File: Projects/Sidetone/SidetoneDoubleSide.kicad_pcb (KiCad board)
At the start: 2 copper layers, 85.5 x 84.8 mm, 54 parts, among them Q1 2N3904, Q2 2N3904, Q3 2N3904, SW1 morse key, SW2 On/off, U1 4N35, U2 LM324, U3 LM386

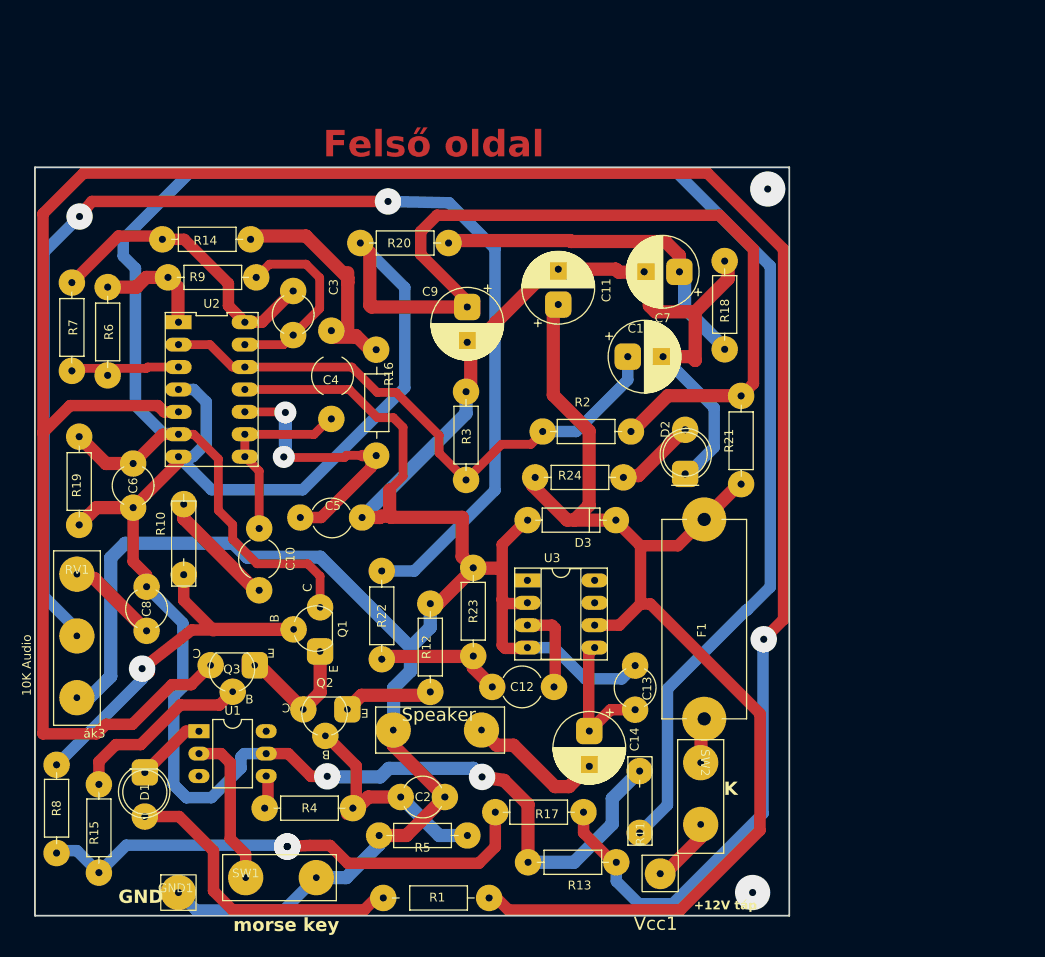
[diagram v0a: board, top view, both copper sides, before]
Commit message: 20240226 sidetone last update
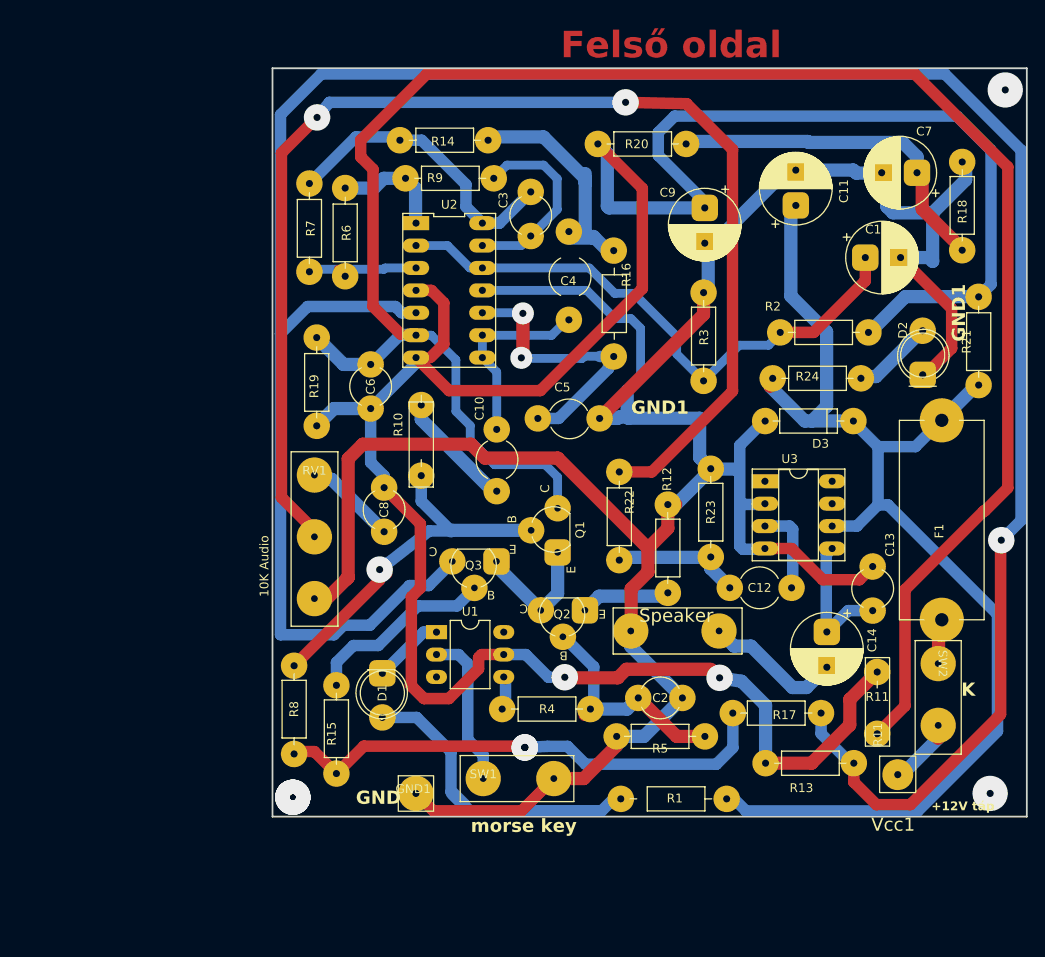
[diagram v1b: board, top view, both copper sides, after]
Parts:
- moved Q3 29.8 mm to (140.3, 107.2)
- moved C11 29.2 mm to (174.3, 66.9)
- moved C12 29.2 mm to (166.8, 110.2)
- moved C14 29.2 mm to (177.8, 115.2)
- moved C2 29.2 mm to (156.4, 122.7)
- moved C9 29.2 mm to (164.0, 67.2)
- moved GND1 29.2 mm to (131.2, 133.5)
- moved R10 29.2 mm to (131.8, 97.5)
- moved R11 29.2 mm to (183.5, 119.8)
- moved R13 29.2 mm to (170.8, 130.1)
- moved R15 29.2 mm to (122.2, 131.3)
- moved R17 29.2 mm to (177.1, 124.4)
- moved R18 29.2 mm to (193.1, 72.0)
- moved R21 29.2 mm to (195.0, 77.2)
- moved R23 29.2 mm to (164.6, 106.7)
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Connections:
- C1 pad 1: Net-(U2A--) -> GNDD
- C10 pad 1: Net-(U2C--) -> GNDD
- C10 pad 2: Net-(C10-Pad2) -> GNDD
- C11 pad 1: Net-(D3-K) -> GNDD
- C12 pad 1: Net-(C12-Pad1) -> GNDD
- C12 pad 2: Net-(U3-+) -> GNDD
- C13 pad 1: Net-(C13-Pad1) -> GNDD
- C14 pad 1: Net-(C13-Pad1) -> GNDD
- C2 pad 1: Net-(Q2-B) -> GNDD
- C3 pad 1: Net-(C3-Pad1) -> GNDD
- C4 pad 1: Net-(U2C--) -> GNDD
- C5 pad 1: Net-(U2C-+) -> GNDD
- C6 pad 1: Net-(Q1-C) -> GNDD
- C6 pad 2: Net-(U2E-V+) -> GNDD
- C7 pad 1: Net-(C7-Pad1) -> GNDD
- C8 pad 1: Net-(U2E-V+) -> GNDD
- C8 pad 2: Net-(C8-Pad2) -> GNDD
- C9 pad 1: Net-(U2E-V+) -> GNDD
- D1 pad 1: Net-(D1-K) -> GNDD
- D1 pad 2: Net-(D1-A) -> GNDD
- D3 pad 1: Net-(D3-K) -> GNDD
- F1 pad 1: Net-(D3-K) -> GNDD
- Q1 pad 2: Net-(Q1-B) -> GNDD
- Q1 pad 3: Net-(Q1-C) -> GNDD
- Q2 pad 1: Net-(Q2-E) -> GNDD
- Q2 pad 2: Net-(Q2-B) -> GNDD
- Q3 pad 2: Net-(Q3-B) -> GNDD
- Q3 pad 3: Net-(Q3-C) -> GNDD
- R1 pad 1: Net-(D1-A) -> GNDD
- R1 pad 2: Net-(D3-K) -> GNDD
- R10 pad 1: Net-(Q1-B) -> GNDD
- R10 pad 2: Net-(C10-Pad2) -> GNDD
- R11 pad 1: Net-(U2E-V+) -> GNDD
- R11 pad 2: Net-(Q1-C) -> GNDD
- R12 pad 1: Net-(Q2-E) -> GNDD
- R13 pad 1: Net-(U2E-V+) -> GNDD
- R13 pad 2: Net-(Q3-C) -> GNDD
- R14 pad 1: Net-(C3-Pad1) -> GNDD
- R15 pad 1: Net-(R15-Pad1) -> GNDD
- R15 pad 2: Net-(Q3-B) -> GNDD
- R16 pad 2: Net-(U2C-+) -> GNDD
- R17 pad 1: Net-(Q3-C) -> GNDD
- R17 pad 2: Net-(R15-Pad1) -> GNDD
- R18 pad 1: Net-(C7-Pad1) -> GNDD
- R19 pad 1: Net-(Q1-C) -> GNDD
- R19 pad 2: Net-(U2E-V+) -> GNDD
- R2 pad 1: Net-(U2E-V+) -> GNDD
- R2 pad 2: Net-(U2A--) -> GNDD
- R20 pad 1: Net-(U2E-V+) -> GNDD
- R20 pad 2: Net-(C7-Pad1) -> GNDD
- R21 pad 1: Net-(U2E-V+) -> GNDD
- R21 pad 2: Net-(D3-K) -> GNDD
- R22 pad 1: Net-(R22-Pad1) -> GNDD
- R22 pad 2: Net-(C12-Pad1) -> GNDD
- R23 pad 1: Net-(C12-Pad1) -> GNDD
- R24 pad 1: Net-(D3-K) -> GNDD
- R3 pad 1: Net-(U2A--) -> GNDD
- R4 pad 2: Net-(Q2-B) -> GNDD
- R5 pad 1: Net-(Q2-B) -> GNDD
- R6 pad 1: Net-(R6-Pad1) -> GNDD
- R6 pad 2: Net-(U2A-+) -> GNDD
- R7 pad 1: Net-(C3-Pad1) -> GNDD
- R7 pad 2: Net-(U2A-+) -> GNDD
- R8 pad 1: Net-(R15-Pad1) -> GNDD
- R8 pad 2: Net-(Q1-B) -> GNDD
- R9 pad 1: Net-(R6-Pad1) -> GNDD
- RV1 pad 1: Net-(C8-Pad2) -> GNDD
- RV1 pad 2: Net-(R22-Pad1) -> GNDD
- SW1 pad 1: Net-(SW1A-A) -> GNDD
- U1 pad 1: Net-(D1-K) -> GNDD
- U1 pad 2: Net-(SW1A-A) -> GNDD
- U1 pad 5: Net-(U2E-V+) -> GNDD
- U2 pad 1: Net-(R6-Pad1) -> GNDD
- U2 pad 10: Net-(U2C-+) -> GNDD
- U2 pad 12: Net-(U2A--) -> GNDD
- U2 pad 14: Net-(C3-Pad1) -> GNDD
- U2 pad 2: Net-(U2A--) -> GNDD
- U2 pad 3: Net-(U2A-+) -> GNDD
- U2 pad 4: Net-(U2E-V+) -> GNDD
- U2 pad 5: Net-(Q3-C) -> GNDD
- U2 pad 6: Net-(Q1-C) -> GNDD
- U2 pad 7: Net-(U2E-V+) -> GNDD
- U2 pad 8: Net-(U2C--) -> GNDD
- U2 pad 9: Net-(U2C--) -> GNDD
- U3 pad 3: Net-(U3-+) -> GNDD
- U3 pad 5: Net-(C13-Pad1) -> GNDD
- U3 pad 6: Net-(D3-K) -> GNDD
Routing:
- net GNDD: track 307.6 -> 1886.3 mm, vias 0 -> 10
- net Net-(U2E-V+): track 288.1 -> 0.00 mm, vias 2 -> 0
- net Net-(Q3-C): track 284.5 -> 0.00 mm, vias 1 -> 0
- net Net-(Q1-C): track 221.6 -> 0.00 mm
- net Net-(R22-Pad1): track 145.2 -> 0.00 mm, vias 2 -> 0
- net Net-(D3-K): track 139.0 -> 0.00 mm
- net Net-(U2A--): track 66.1 -> 0.00 mm
- net Net-(R15-Pad1): track 58.1 -> 0.00 mm, vias 2 -> 0
- net Net-(Q1-B): track 42.2 -> 0.00 mm, vias 1 -> 0
- net Net-(C7-Pad1): track 39.7 -> 0.00 mm
- net Net-(D1-A): track 35.0 -> 0.00 mm
- net Net-(C3-Pad1): track 34.3 -> 0.00 mm
- net Net-(U2C-+): track 32.9 -> 0.00 mm, vias 2 -> 0
- net Net-(Q2-B): track 26.1 -> 0.00 mm
- net Net-(U2C--): track 22.0 -> 0.00 mm
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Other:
- board text added: "GND1"
- board text added: "R11"
- board text removed: "ák3"
